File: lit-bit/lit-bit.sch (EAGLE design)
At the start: 16 parts, among them IC1 ATMEGA32U4-MU, U1 S-1317A33-M5T1U4, U2 32U4, U3 MCP73831T, Y1 8MHz

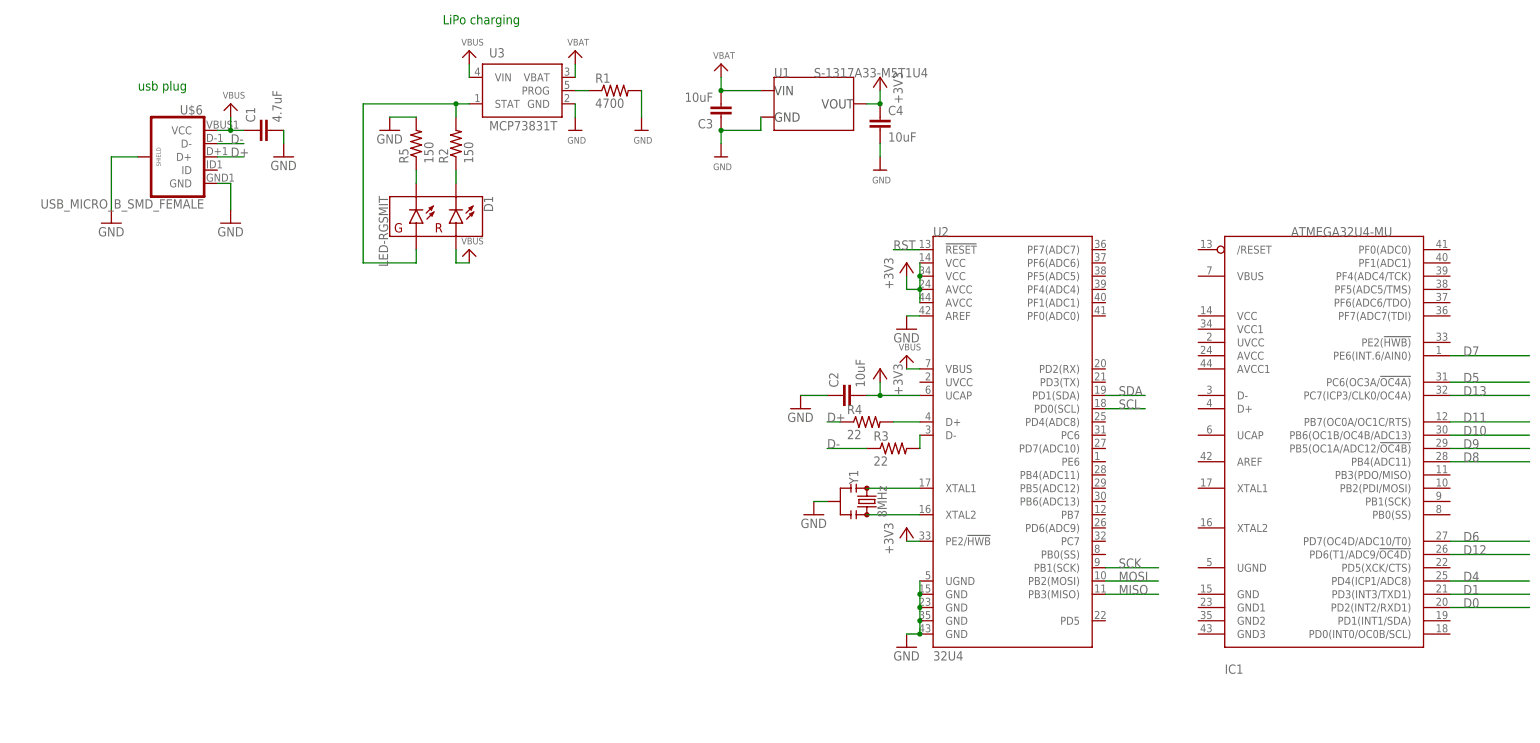
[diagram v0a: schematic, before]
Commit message: removed QFN 32u4
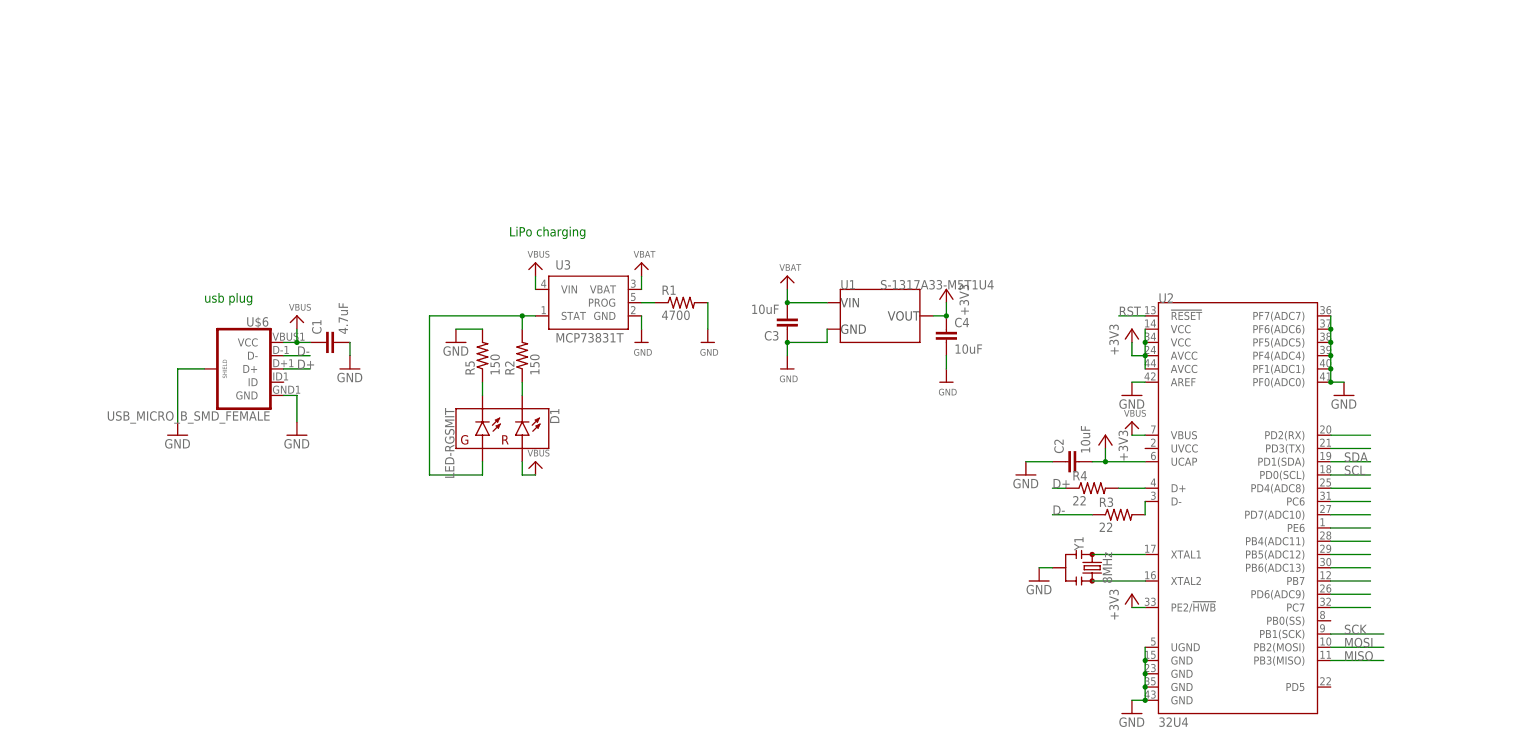
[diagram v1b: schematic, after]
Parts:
- removed IC1: ATMEGA32U4-MU, microbuilder:ATMEGA32U4-MU
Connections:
- removed net D0: IC1.PD2(INT2/RXD1)
- removed net D1: IC1.PD3(INT3/TXD1)
- removed net D10: IC1.PB6(OC1B/OC4B/ADC13)
- removed net D11: IC1.PB7(OC0A/OC1C/RTS)
- removed net D12: IC1.PD6(T1/ADC9/!OC4D)
- removed net D13: IC1.PC7(ICP3/CLK0/OC4A)
- removed net D4: IC1.PD4(ICP1/ADC8)
- removed net D5: IC1.PC6(OC3A/!OC4A)
- removed net D6: IC1.PD7(OC4D/ADC10/T0)
- removed net D7: IC1.PE6(INT.6/AIN0)
- removed net D8: IC1.PB4(ADC11)
- removed net D9: IC1.PB5(OC1A/ADC12/!OC4B)
- new net N$10: U2.PB7
- new net N$11: U2.PB6(ADC13)
- new net N$12: U2.PB5(ADC12)
- new net N$13: U2.PB4(ADC11)
- new net N$14: U2.PD7(ADC10)
- new net N$15: U2.PD3(TX)
- new net N$16: U2.PD2(RX)
- new net N$17: U2.PD6(ADC9)
- new net N$18: U2.PC7
- new net N$19: U2.PD4(ADC8)
- new net N$8: U2.PE6
- new net N$9: U2.PC6
- net GND: now also U2.PF0(ADC0), U2.PF1(ADC1), U2.PF4(ADC4), U2.PF5(ADC5), U2.PF6(ADC6), U2.PF7(ADC7)
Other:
- moved on the sheet: C1, C2, C3, C4, D1, R1, R2, R3, R4, R5, U$6, U1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
